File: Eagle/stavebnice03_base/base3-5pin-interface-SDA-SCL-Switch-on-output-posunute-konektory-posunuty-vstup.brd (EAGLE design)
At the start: 16 parts

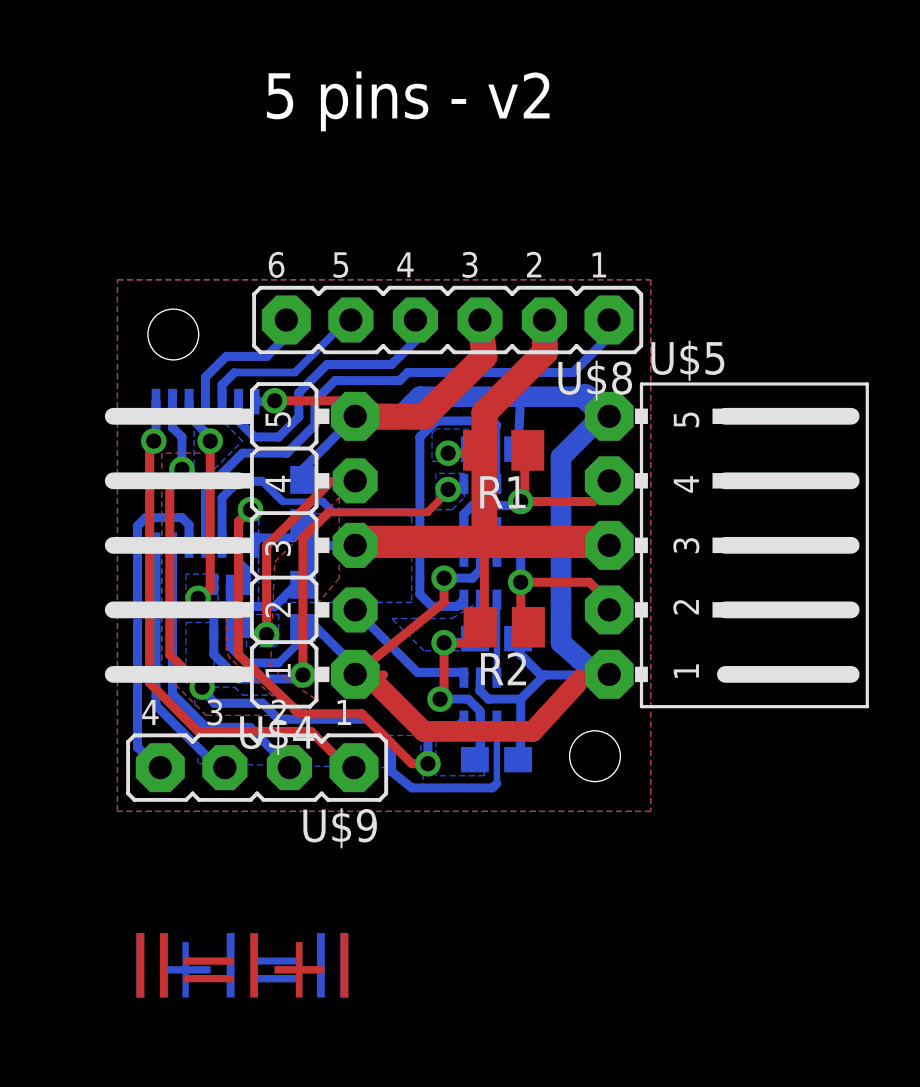
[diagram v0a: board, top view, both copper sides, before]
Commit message: minor changes
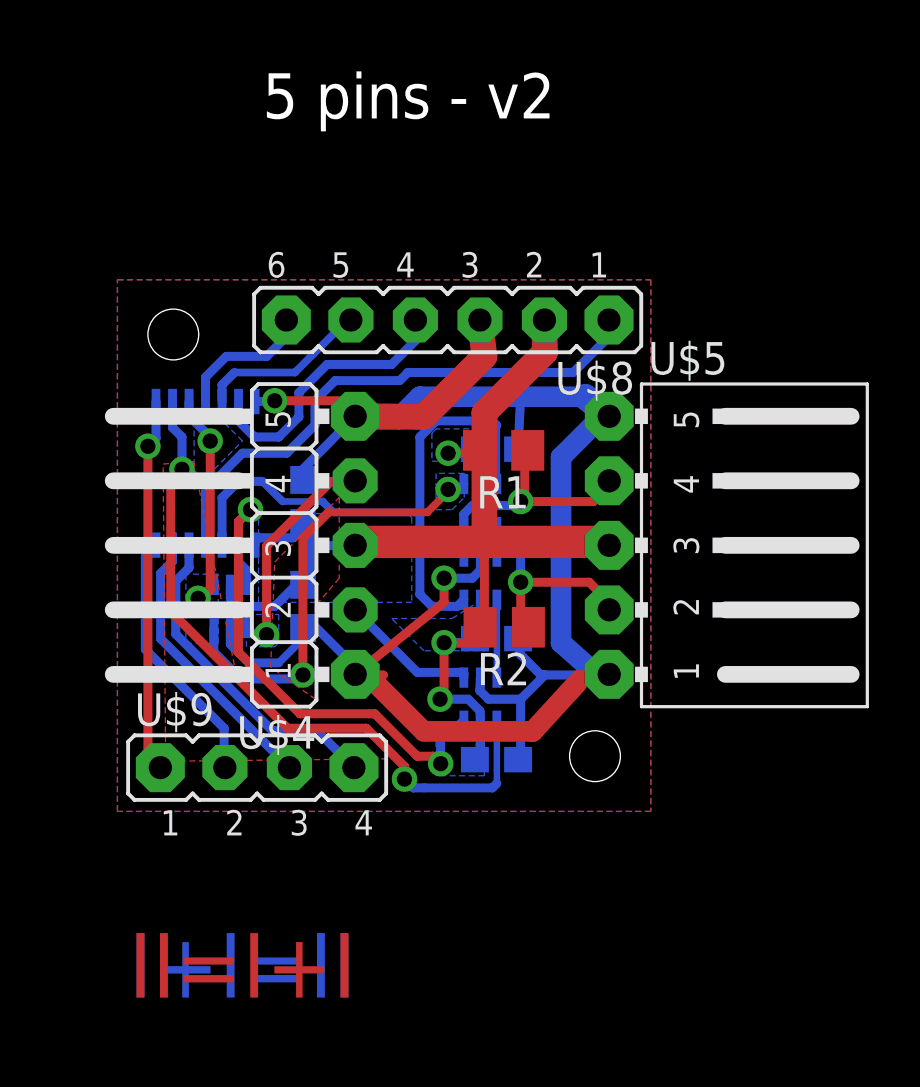
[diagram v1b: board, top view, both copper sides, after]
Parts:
- turned U$9 to 0 degrees
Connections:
- removed net N$16: U$1.7, U$9.3
- new net N$3: U$1.7, U$9.2
- net N$17: now also U$9.3; no longer U$9.2
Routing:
- net N$3: track 0.00 -> 10.2 mm
- net N$16: track 10.0 -> 0.00 mm
- net N$18: track 21.0 -> 14.7 mm
- net N$4: track 28.5 -> 27.1 mm
- net N$17: track 11.7 -> 11.1 mm
- removed copper zone on layer 16, net N$4
